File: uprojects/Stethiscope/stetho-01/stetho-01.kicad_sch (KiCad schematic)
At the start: 2 parts, among them U1 ESP32-S3-WROOM-1-N16R8, U2 ADS1298IPAGR

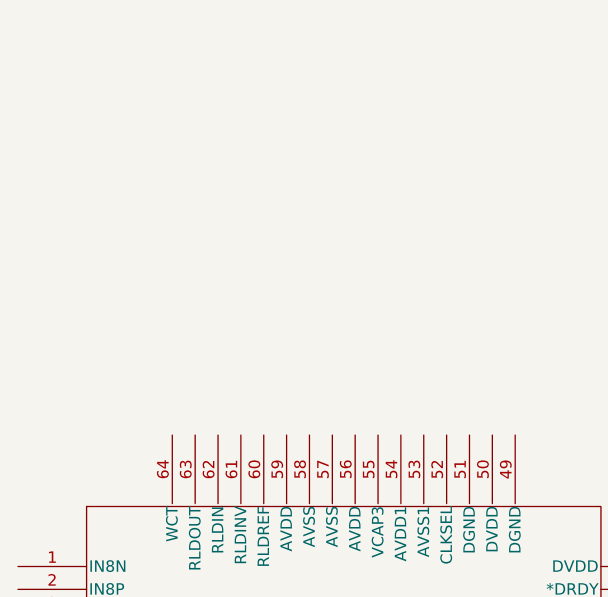
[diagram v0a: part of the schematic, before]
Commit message: Update 11 May 2026
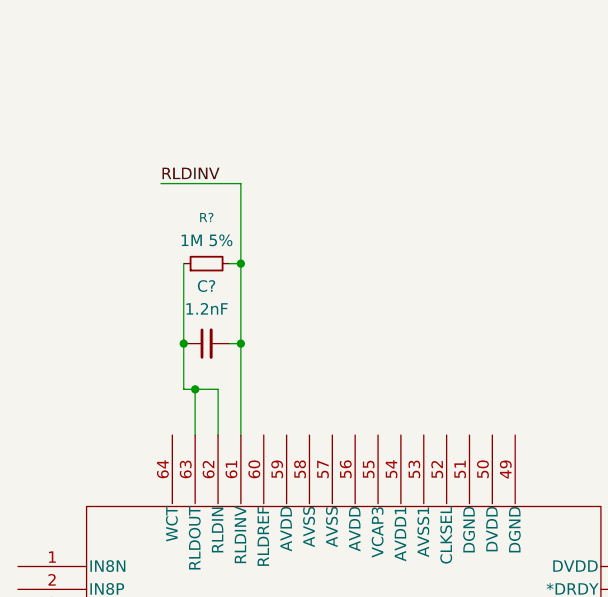
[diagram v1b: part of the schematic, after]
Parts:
- added C?: 1.2nF, symbol Device:C_Small
- added R?: 1M 5%, symbol Device:R_Small
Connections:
- net RLDINV: now reaches U2.61 (RLDINV)
- net RLDINV: now also C?.2, R?.2
- net at U2.62 (RLDIN): now also U2.63 (RLDOUT), C?.1, R?.1
